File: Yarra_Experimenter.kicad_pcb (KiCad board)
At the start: 2 copper layers, 70 x 35 mm, 146 parts

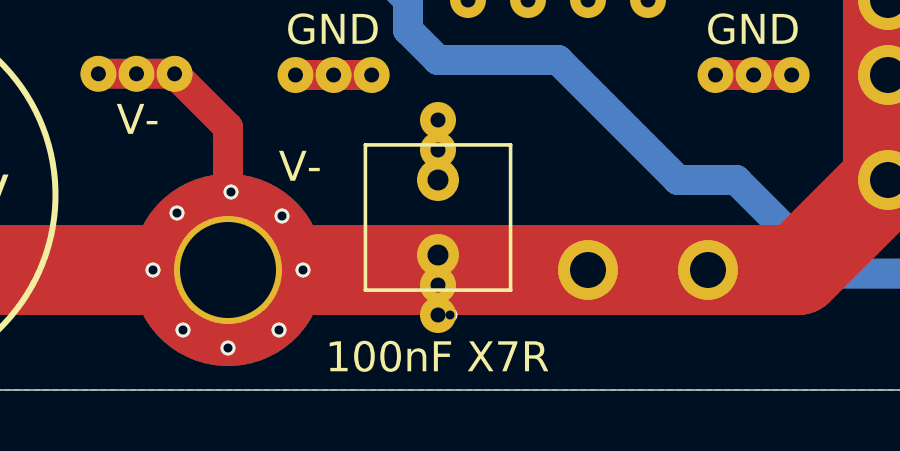
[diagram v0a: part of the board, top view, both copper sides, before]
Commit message: Saved
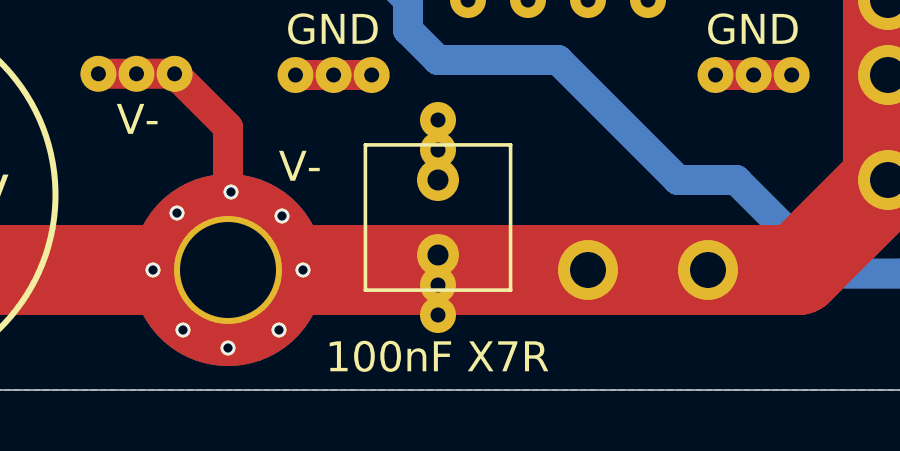
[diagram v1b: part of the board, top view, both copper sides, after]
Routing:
- net Net-(C1-Pad2): vias 9 -> 8
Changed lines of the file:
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@@
     (thickness 1.6)
     (drawings 31)
-    (tracks 131)
+    (tracks 130)
     (zones 0)
     (modules 146)
@@
   (segment (start 104 41.5) (end 104 43.5) (width 1) (layer F.Cu) (net 3))
   (segment (start 81.25 64.5) (end 83.79 64.5) (width 1) (layer F.Cu) (net 3))
-  (via (at 86.4 72.5) (size 0.5) (drill 0.3) (layers F.Cu B.Cu) (net 4))
   (via (at 79 73.6) (size 0.5) (drill 0.3) (layers F.Cu B.Cu) (net 4))
   (via (at 79.1 68.4) (size 0.5) (drill 0.3) (layers F.Cu B.Cu) (net 4))
